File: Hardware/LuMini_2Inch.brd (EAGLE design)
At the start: 54.1 x 54.1 mm, 64 parts, among them J1 DOUBLE_LED_PAD, J2 DOUBLE_LED_PAD, J3 DOUBLE_LED_PAD

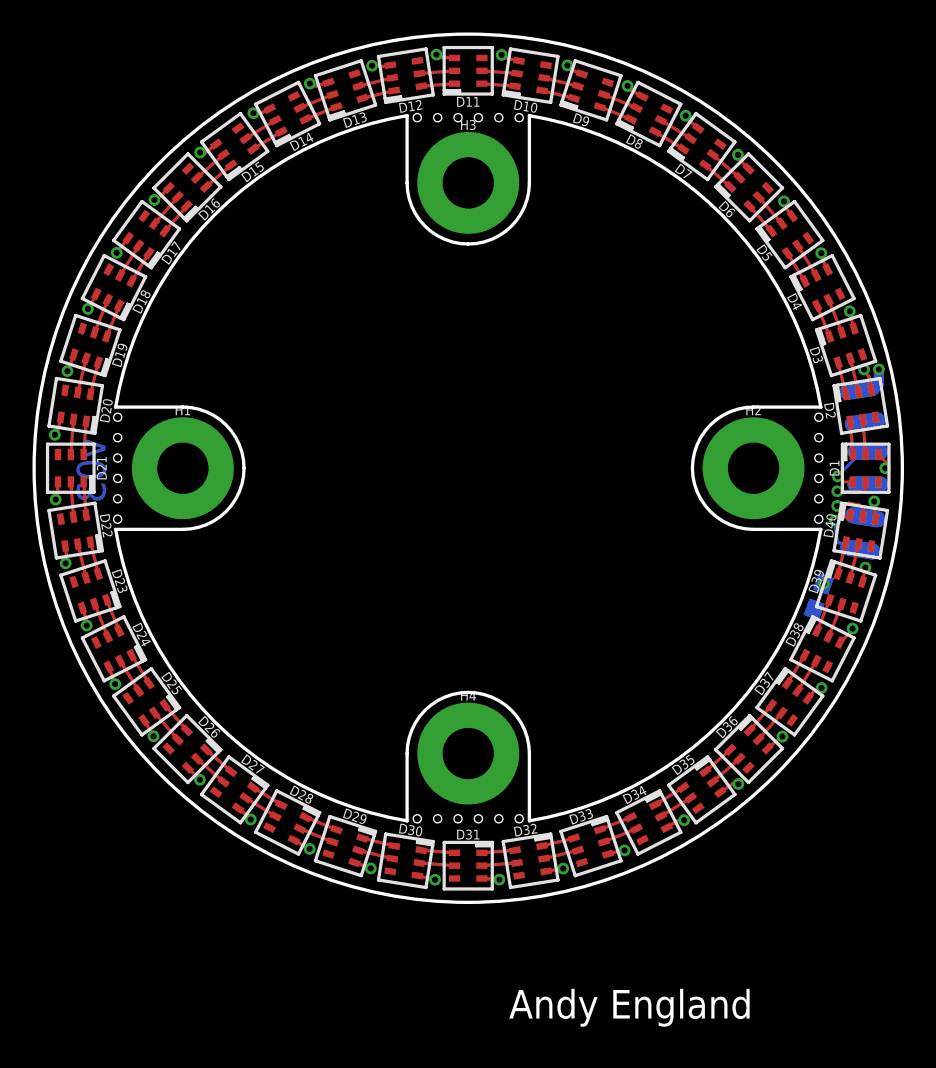
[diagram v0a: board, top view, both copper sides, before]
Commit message: post checklist
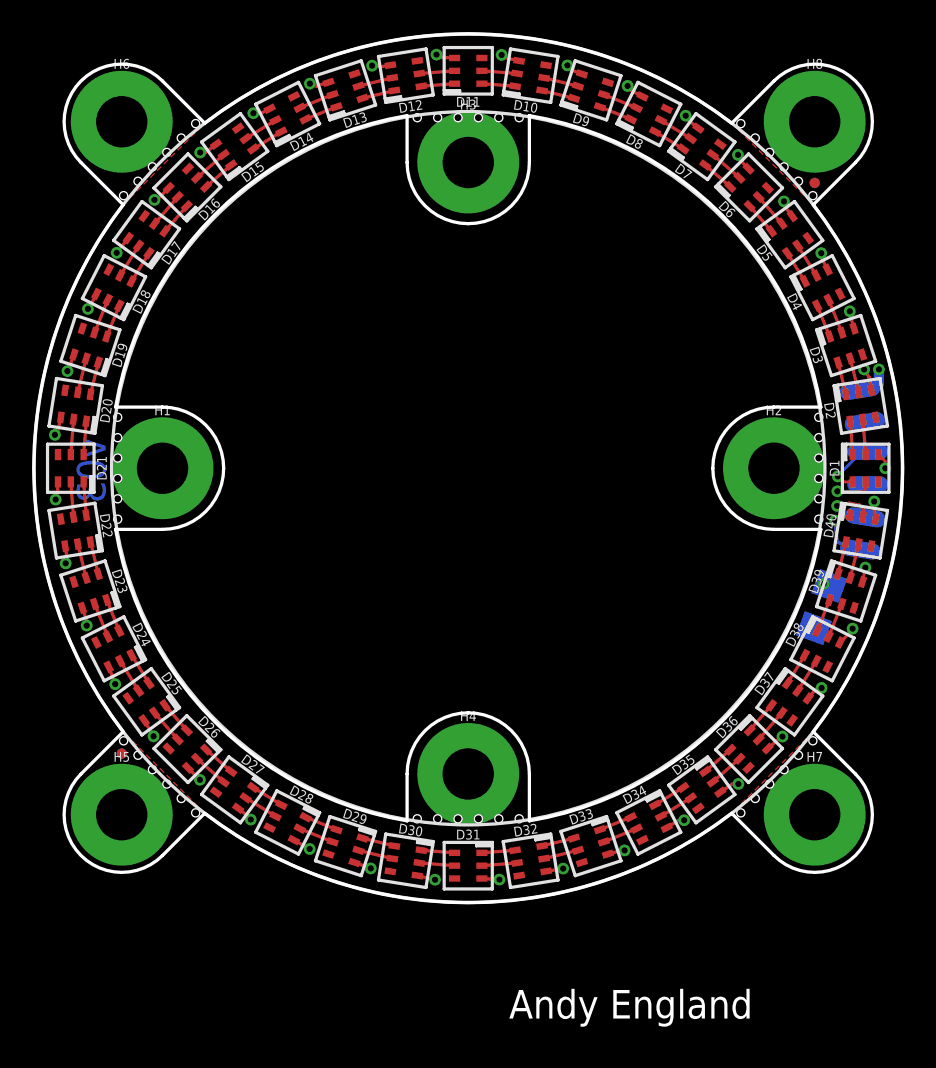
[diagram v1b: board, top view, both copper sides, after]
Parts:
- added FD1, FD2, FD3, FD4: FIDUCIALUFIDUCIAL, SparkFun-Aesthetics:FIDUCIAL-MICRO
- added H5, H6, H7, H8: STANDOFF_ELECTRICALSTANDOFF-ELECTRICAL-NOTHERMALS, SparkFun-Hardware:STANDOFF-ELECTRICAL-NOTHERMALS
- added U$14: (no value), SparkFun-Aesthetics:ORDERING_INSTRUCTIONS
- C1: value 4.7uF -> DNP; device SparkFun-Capacitors:0603 -> SparkFun-Capacitors:1206
- U$1: device buzzard_labels (2):LUMINI0 -> buzzard_labels (8):LUMINI_2#0
- moved H2 1.27 mm to (47.0, 27.9)
- moved H3 1.27 mm to (27.9, 47.0)
- moved H1 1.27 mm to (8.89, 27.9)
- moved H4 1.27 mm to (27.9, 8.89)
- moved U$1 0.89 mm to (23.8, 3.40)
- moved C1 0.67 mm to (50.0, 19.3)
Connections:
- net GND: now also H5.P1, H6.P1, H7.P1, H8.P1
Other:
- board size 54.1 x 54.1 mm -> 54.2 x 54.2 mm
- board text added: "Black PCB 2 Oz. Cu"
